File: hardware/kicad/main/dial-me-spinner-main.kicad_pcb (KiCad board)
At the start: 4 copper layers, 64 x 64 mm, 209 parts, among them J1 LINK, J10 SWD, J11 NFC_COIL, J20 OLED_ZIF30, J40 MOTOR, U1 RT9080-33GJ5, U10 MDBT50Q-U1MV2, U11 W25Q128JVSIQ, U12 USBLC6-2SC6, U2 TPS22917DBVR, U20 TPS61040DBVR, U21 TPS22917DBVR, U30 TMAG5273A2QDBVR, U31 LIS2DW12TR, U32 TPD4E05U06DQAR, U40 DRV8837DSGR, U41 DRV8837DSGR, U42 DRV5032FADBZR, U43 SN74LV1T34DBVR, Y1 32.768k 9pF

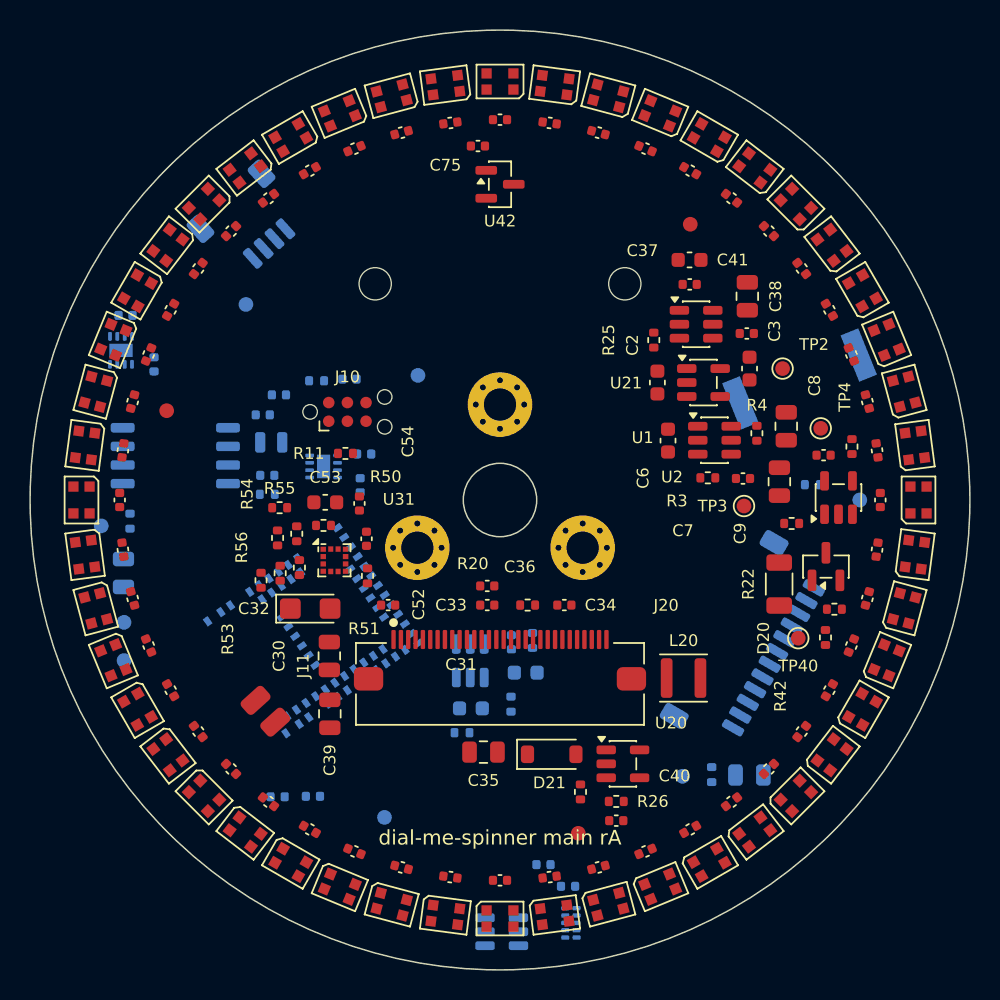
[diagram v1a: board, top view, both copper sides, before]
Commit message: WIP: main board routing (attempt 2 in progress)
Co-Authored-By: Claude Opus 5.5 <noreply@anthropic.com>
Claude-Session: https://claude.ai/code/session_01P3cqdBhxLcWY3sGUVf9LAJ
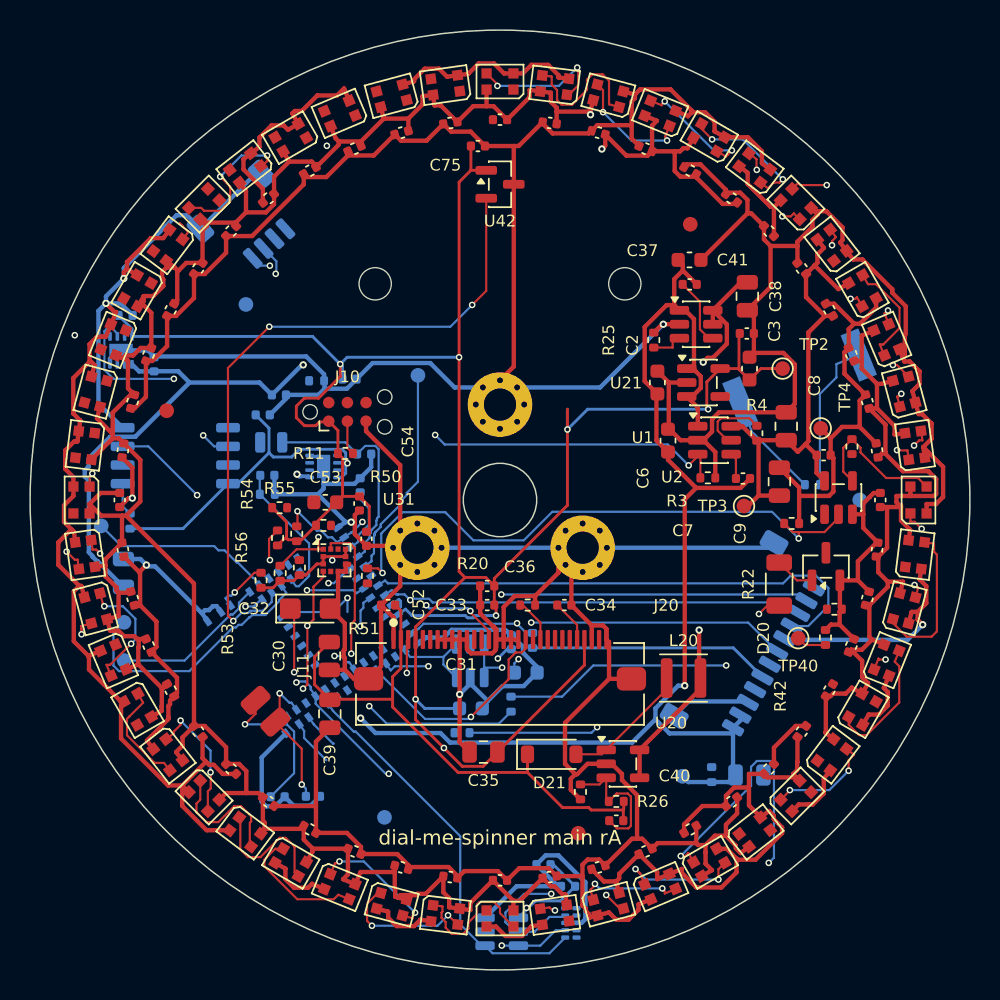
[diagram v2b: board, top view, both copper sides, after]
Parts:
- turned C106 to 128 degrees
- turned C132 to -37 degrees
- turned C142 to 38 degrees
- turned C144 to 53 degrees
- turned C118 to -142 degrees
- turned C120 to -127 degrees
- turned C108 to 143 degrees
- turned C130 to -52 degrees
- turned D140 to 23 degrees
- turned D146 to 68 degrees
- turned D104 to 113 degrees
- turned D134 to -22 degrees
- turned D110 to 158 degrees
- turned D128 to -67 degrees
- turned D116 to -157 degrees
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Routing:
- net GND: track 0.00 -> 758.8 mm, vias 0 -> 8
- net VLED: track 0.00 -> 332.9 mm, vias 0 -> 2
- net +3V3: track 0.00 -> 225.7 mm, vias 0 -> 11
- net VSYS: track 0.00 -> 146.5 mm, vias 0 -> 4
- net I2C_SDA: track 0.00 -> 64.3 mm, vias 0 -> 4
- net HOME_N: track 0.00 -> 47.2 mm, vias 0 -> 3
- net TMAG_INT_N: track 0.00 -> 47.1 mm, vias 0 -> 3
- net LED_PWR_EN: track 0.00 -> 41.7 mm, vias 0 -> 3
- net /LED ring/LED_DIN_R: track 0.00 -> 40.3 mm, vias 0 -> 2
- net I2C_SCL: track 0.00 -> 39.9 mm, vias 0 -> 1
- net OLED_VIN: track 0.00 -> 39.1 mm, vias 0 -> 2
- net +13V_OLED: track 0.00 -> 37.6 mm
- net MOT_B_IN1: track 0.00 -> 31.1 mm, vias 0 -> 2
- net TMAG_SDA: track 0.00 -> 29.0 mm, vias 0 -> 3
- net TMAG_SCL: track 0.00 -> 27.2 mm
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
